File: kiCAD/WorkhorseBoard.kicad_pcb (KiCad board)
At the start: 4 copper layers, 205 x 97 mm, 384 parts, among them J1 USB_B_Mini, J10 MAIN_POWER, J11 BED_POWER, J12 H0, J13 F0, J15 F1, J16 F4, J17 H1, J19 F2, J2 Micro_SD_Card, J20 F5, J21 H2, J22 F3, J23 HB, J24 Conn_01x02, J25 Conn_01x02, J26 Conn_01x02, J27 Conn_01x02, J28 Conn_01x03, J29 Conn_01x03, J3 Conn_01x06, J30 Conn_01x03, J31 Conn_01x03, J32 Conn_01x03, J33 Conn_01x03, J4 X, J5 E0, J6 Y, J7 E1, J8 Z, J9 E2, Q1 Q_NMOS_GSD, Q10 Q_NMOS_GDS, Q2 Q_NMOS_GDS, Q3 Q_NMOS_GSD, Q4 Q_NMOS_GSD, Q5 Q_NMOS_GDS, Q6 Q_NMOS_GSD, Q7 Q_NMOS_GSD, Q8 Q_NMOS_GDS, Q9 Q_NMOS_GSD, SW1 SW_Push, U1 24C02, U10 TPS54531, U11 TPS54531, U12 AP7361C-33E-13, U13 74HCT365, U14 74HCT365, U2 USBLC6-2SC6, U3 STM32F446VETx, U4 TMC2209, U5 TMC2209, U6 TMC2209, U7 TMC2209, U8 TMC2209, U9 TMC2209, Y1 X322512MSB4SI

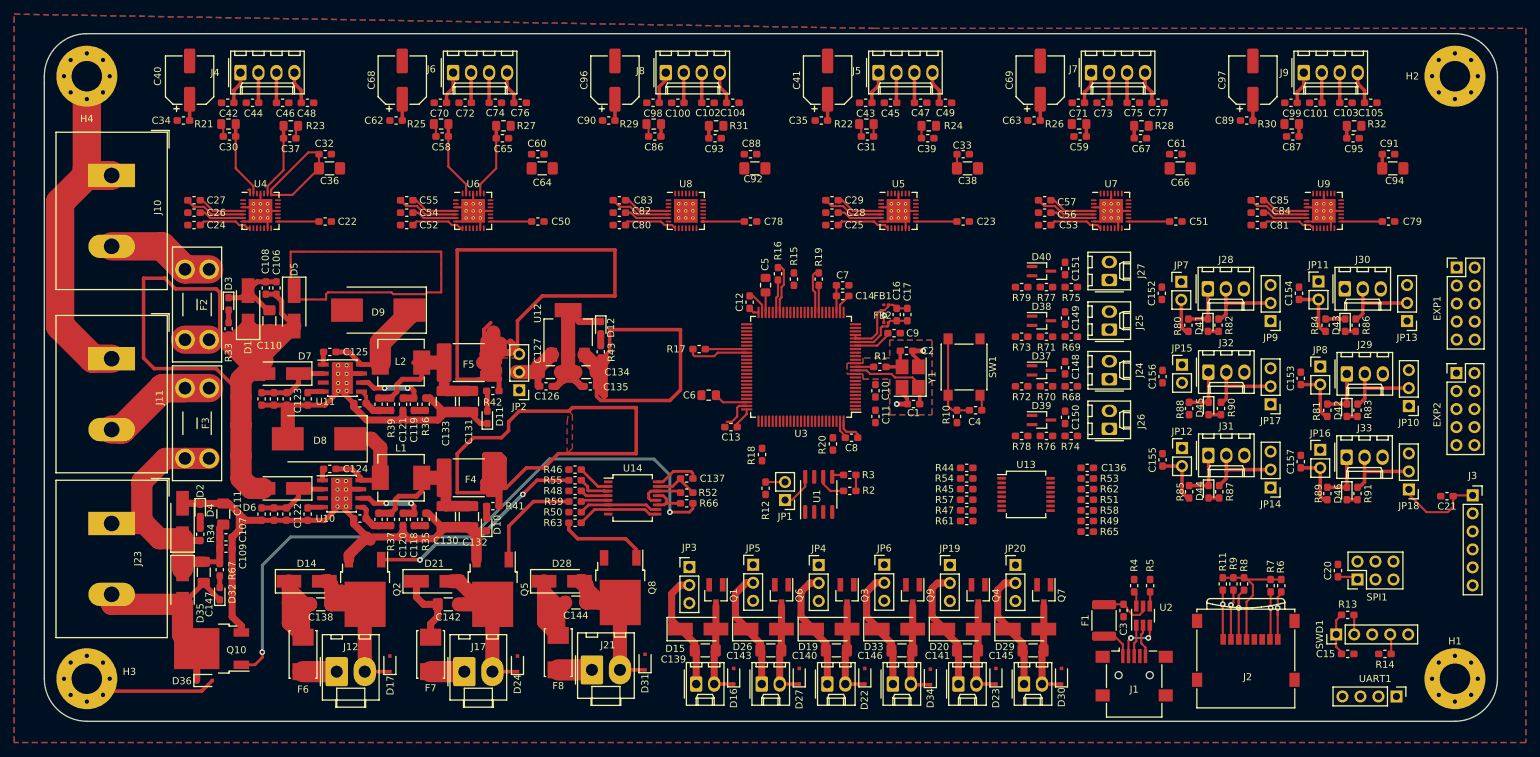
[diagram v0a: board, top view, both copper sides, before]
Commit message: small changes.
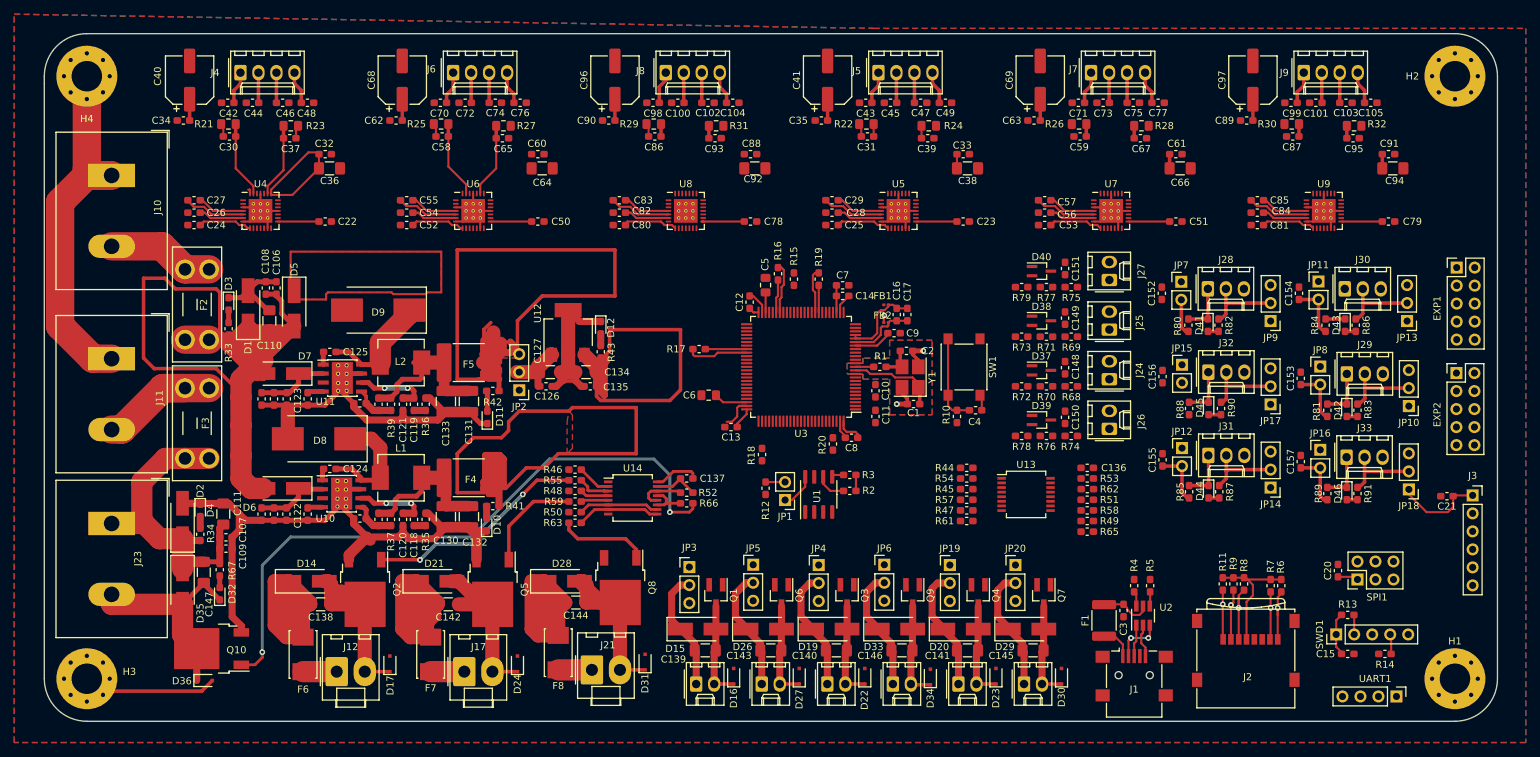
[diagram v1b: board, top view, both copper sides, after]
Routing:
- net +24V: track 173.6 -> 248.9 mm
- net VM: track 96.4 -> 98.4 mm
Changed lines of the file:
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@@
     (thickness 1.6)
     (drawings 9)
-    (tracks 1137)
+    (tracks 1172)
     (zones 0)
     (modules 384)
@@
   (segment (start 166.5 41.25) (end 166.5 38.25) (width 0.5) (layer F.Cu) (net 15))
   (segment (start 196.5 41.25) (end 196.5 38.25) (width 0.5) (layer F.Cu) (net 15))
+  (segment (start 184.75 48) (end 184.75 46) (width 0.5) (layer F.Cu) (net 15))
   (segment (start 54.05 54) (end 49.812986 54) (width 0.3) (layer F.Cu) (net 16))
   (segment (start 48.312986 52.5) (end 48 52.5) (width 0.3) (layer F.Cu) (net 16))
@@
   (segment (start 59.5 68.5) (end 61.25 70.25) (width 0.7) (layer F.Cu) (net 49))
   (segment (start 59.5 66.75) (end 59.5 68.5) (width 0.7) (layer F.Cu) (net 49))
-  (segment (start 78.5 108.5) (end 78.5 106.25) (width 1) (layer F.Cu) (net 49))
   (segment (start 81.5 109.5) (end 79.5 109.5) (width 1) (layer F.Cu) (net 49))
   (segment (start 79.5 109.5) (end 78.5 108.5) (width 1) (layer F.Cu) (net 49))
@@
   (segment (start 41.5 76.25) (end 50.25 76.25) (width 0.5) (layer F.Cu) (net 49))
   (segment (start 50.25 76.25) (end 53.75 79.75) (width 0.5) (layer F.Cu) (net 49))
+  (segment (start 79.5 113.14) (end 80.5 114.14) (width 2) (layer F.Cu) (net 49))
+  (segment (start 79.5 109.5) (end 79.5 109.75) (width 2) (layer F.Cu) (net 49))
+  (segment (start 79.5 109.75) (end 80.25 110.5) (width 2) (layer F.Cu) (net 49))
+  (segment (start 80.25 111) (end 79.5 111.75) (width 2) (layer F.Cu) (net 49))
+  (segment (start 80.25 110.5) (end 80.25 111) (width 2) (layer F.Cu) (net 49))
+  (segment (start 79.5 111.75) (end 79.5 113.14) (width 2) (layer F.Cu) (net 49))
+  (segment (start 80.75 109.5) (end 78.5 107.25) (width 2) (layer F.Cu) (net 49))
+  (segment (start 78.5 108.5) (end 78.5 107.25) (width 1) (layer F.Cu) (net 49))
+  (segment (start 81.5 109.5) (end 80.75 109.5) (width 2) (layer F.Cu) (net 49))
+  (segment (start 78.5 107.25) (end 78.5 106.25) (width 1) (layer F.Cu) (net 49))
+  (segment (start 99.5 109.25) (end 96.5 106.25) (width 2) (layer F.Cu) (net 49))
+  (segment (start 63.5 109.25) (end 60.5 106.25) (width 2) (layer F.Cu) (net 49))
+  (segment (start 63.5 109.5) (end 63.5 109.25) (width 2) (layer F.Cu) (net 49))
+  (segment (start 81.5 109.25) (end 78.5 106.25) (width 2) (layer F.Cu) (net 49))
+  (segment (start 81.5 109.5) (end 81.5 109.25) (width 2) (layer F.Cu) (net 49))
+  (segment (start 98.5 113.89) (end 95.64 113.89) (width 2) (layer F.Cu) (net 49))
+  (segment (start 95.64 113.89) (end 94.75 113) (width 2) (layer F.Cu) (net 49))
+  (segment (start 94.75 113) (end 94.75 106.25) (width 2) (layer F.Cu) (net 49))
+  (segment (start 94.75 106.25) (end 96.5 106.25) (width 2) (layer F.Cu) (net 49))
+  (segment (start 76.5 106.25) (end 78.5 106.25) (width 2) (layer F.Cu) (net 49))
+  (segment (start 76.5 108.25) (end 77.25 108.25) (width 2) (layer F.Cu) (net 49))
+  (segment (start 76.5 108.25) (end 76.5 106.25) (width 2) (layer F.Cu) (net 49))
+  (segment (start 77.25 108.25) (end 78.75 109.75) (width 2) (layer F.Cu) (net 49))
+  (segment (start 78.75 109.75) (end 78.75 110.75) (width 2) (layer F.Cu) (net 49))
+  (segment (start 78.75 110.75) (end 78.25 111.25) (width 2) (layer F.Cu) (net 49))
+  (segment (start 77.64 114.14) (end 76.5 113) (width 2) (layer F.Cu) (net 49))
+  (segment (start 80.5 114.14) (end 77.64 114.14) (width 2) (layer F.Cu) (net 49))
+  (segment (start 76.5 113) (end 76.5 108.25) (width 2) (layer F.Cu) (net 49))
+  (segment (start 80.5 114.14) (end 79.89 114.14) (width 2) (layer F.Cu) (net 49))
+  (segment (start 78.5 112.75) (end 78.5 106.25) (width 2) (layer F.Cu) (net 49))
+  (segment (start 79.89 114.14) (end 78.5 112.75) (width 2) (layer F.Cu) (net 49))
+  (segment (start 62.5 114.14) (end 60.14 114.14) (width 2) (layer F.Cu) (net 49))
+  (segment (start 60.14 114.14) (end 58.5 112.5) (width 2) (layer F.Cu) (net 49))
+  (segment (start 58.5 112.5) (end 58.5 106.25) (width 2) (layer F.Cu) (net 49))
+  (segment (start 58.5 106.25) (end 60.5 106.25) (width 2) (layer F.Cu) (net 49))
   (segment (start 35.5 98.1) (end 40.1 98.1) (width 3) (layer F.Cu) (net 50))
   (segment (start 42.25 100.25) (end 45.5 100.25) (width 3) (layer F.Cu) (net 50))
@@
       )
     )
+  )
+  (zone (net 49) (net_name +24V) (layer F.Cu) (hatch edge 0.508)
+    (connect_pads (clearance 0.508))
+    (min_thickness 0.254)
+    (fill yes (arc_segments 32) (thermal_gap 0.508) (thermal_bridge_width 0.508))
+    (polygon
+      (pts
+        (xy 80 109.25) (xy 79.25 114.25) (xy 77.5 114.25) (xy 76.25 112.75) (xy 76.5 106.5)
+        (xy 79.25 106.5)
+      )
+    )
